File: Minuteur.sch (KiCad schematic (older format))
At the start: 44 parts, among them J1 Screw_Terminal_01x02, J2 ICSP, J3 piezo, J4 Conn_01x10, J5 output, J6 Screw_Terminal_01x03, Q1 BC818, SW1 Rotary_Encoder_Switch, SW2 SW_Push_SPDT_2Leds, U1 ATmega328P-AU, U2 LD1117S50TR_SOT223, U3 MAX7219, U4 PC817, U5 CC56-12EWA, Y1 16MHz

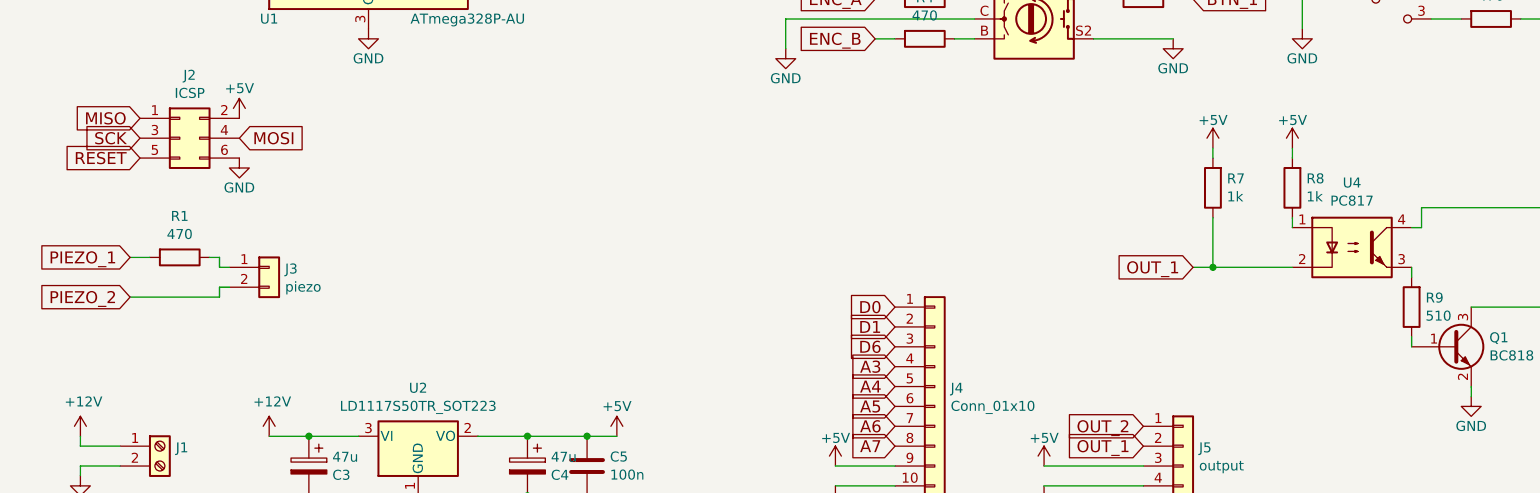
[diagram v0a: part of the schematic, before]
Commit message: All routing done, DRC ok.
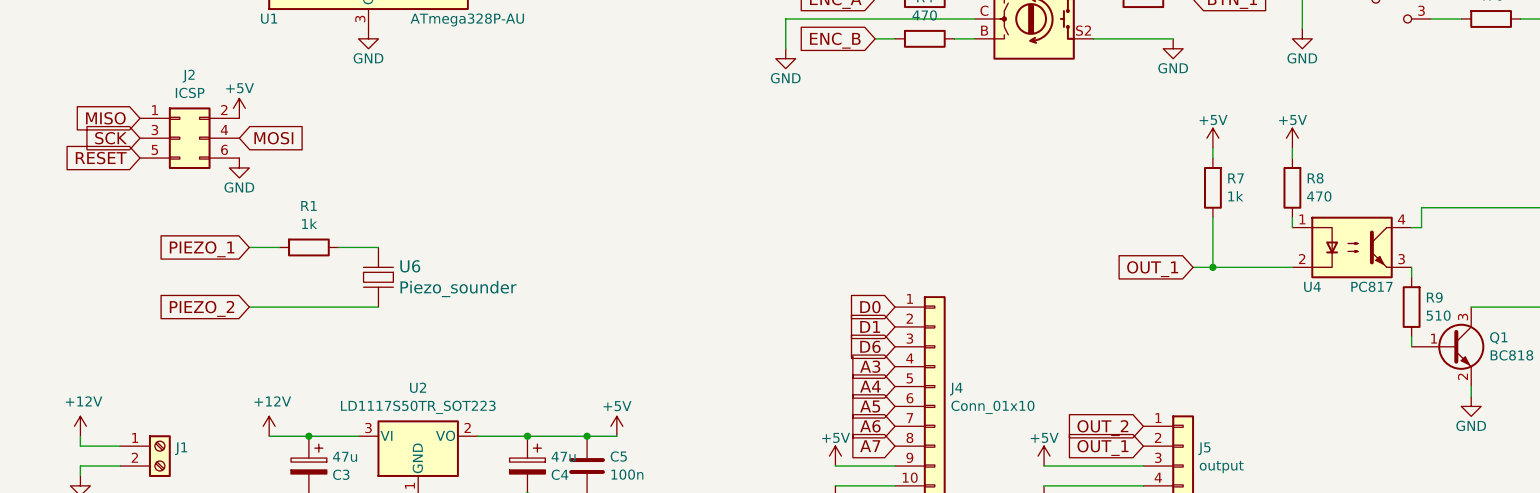
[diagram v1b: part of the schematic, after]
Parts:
- removed J3: piezo, Connector_PinHeader_2.54mm:PinHeader_1x02_P2.54mm_Vertical, symbol Connector_Generic:Conn_01x02
- added U6: Piezo_sounder, IC_Perso:Murata_PKMCS0909_xxxxx, symbol Chip_Perso:Piezo_sounder
- R1: value 470 -> 1k
- R8: value 1k -> 470
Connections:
- net PIEZO_2: now also U6.2
- net at R1.1: now also U6.1
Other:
- moved on the sheet: R1
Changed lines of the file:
@@
 Text GLabel 3150 1700 2    60   Input ~ 0
 PIEZO_2
-Text GLabel 1350 5450 0    60   Input ~ 0
+Text GLabel 1950 5400 0    60   Input ~ 0
 PIEZO_1
 Text GLabel 3150 3700 2    60   Input ~ 0
@@
 	1    0    0    -1
 $EndComp
-Text GLabel 1350 5650 0    60   Input ~ 0
+Text GLabel 1950 5700 0    60   Input ~ 0
 PIEZO_2
 Wire Wire Line
@@
 Wire Wire Line
 	4950 2200 4950 2550
-Wire Wire Line
-	1350 5650 1800 5650
-Wire Wire Line
-	1800 5650 1800 5600
-Wire Wire Line
-	1800 5600 1850 5600
-Wire Wire Line
-	1350 5450 1450 5450
-Wire Wire Line
-	1750 5450 1800 5450
-Wire Wire Line
-	1800 5450 1800 5500
-Wire Wire Line
-	1800 5500 1850 5500
 Text GLabel 3150 1800 2    60   Input ~ 0
 PIEZO_1
@@
 P 7200 5100
 F 0 "R8" H 7130 5054 50  0000 R CNN
-F 1 "1k" H 7130 5145 50  0000 R CNN
+F 1 "470" H 7130 5145 50  0000 R CNN
 F 2 "Resistor_SMD:R_0805_2012Metric" V 7130 5100 50  0001 C CNN
 F 3 "~" H 7200 5100 50  0001 C CNN
@@
 Connection ~ 9100 5200
 $Comp
-L Device:R R1
-U 1 1 5EF81C42
-P 1600 5450
-F 0 "R1" V 1393 5450 50  0000 C CNN
-F 1 "470" V 1484 5450 50  0000 C CNN
-F 2 "Resistor_SMD:R_0805_2012Metric" V 1530 5450 50  0001 C CNN
-F 3 "~" H 1600 5450 50  0001 C CNN
-	1    1600 5450
-	0    1    1    0
-$EndComp
-$Comp
 L Device:C C5
 U 1 1 5EF86361
@@
 U 1 1 5EFADC83
 P 7500 5400
-F 0 "U4" H 7500 5725 50  0000 C CNN
-F 1 "PC817" H 7500 5634 50  0000 C CNN
+F 0 "U4" H 7300 5200 50  0000 C CNN
+F 1 "PC817" H 7600 5200 50  0000 C CNN
 F 2 "Package_DIP:DIP-4_W7.62mm" H 7300 5200 50  0001 L CIN
 F 3 "http://www.soselectronic.cz/a_info/resource/d/pc817.pdf" H 7500 5400 50  0001 L CNN
@@
 	1050 1600 1350 1600
 $Comp
-L Connector_Generic:Conn_01x02 J3
-U 1 1 5EFB8BD6
-P 2050 5500
-F 0 "J3" H 2130 5492 50  0000 L CNN
-F 1 "piezo" H 2130 5401 50  0000 L CNN
-F 2 "Connector_PinHeader_2.54mm:PinHeader_1x02_P2.54mm_Vertical" H 2050 5500 50  0001 C CNN
-F 3 "~" H 2050 5500 50  0001 C CNN
-	1    2050 5500
-	1    0    0    -1
+L Device:R R1
+U 1 1 5EF81C42
+P 2250 5400
+F 0 "R1" V 2043 5400 50  0000 C CNN
+F 1 "1k" V 2134 5400 50  0000 C CNN
+F 2 "Resistor_SMD:R_0805_2012Metric" V 2180 5400 50  0001 C CNN
+F 3 "~" H 2250 5400 50  0001 C CNN
+	1    2250 5400
+	0    1    1    0
+$EndComp
+Wire Wire Line
+	2400 5400 2600 5400
+Wire Wire Line
+	1950 5700 2600 5700
+Wire Wire Line
+	2100 5400 1950 5400
+$Comp
+L Chip_Perso:Piezo_sounder U6
+U 1 1 5FCD1C61
+P 2600 5550
+F 0 "U6" V 2547 5653 60  0000 L CNN
+F 1 "Piezo_sounder" V 2653 5653 60  0000 L CNN
+F 2 "IC_Perso:Murata_PKMCS0909_xxxxx" H 2600 5550 60  0001 C CNN
+F 3 "https://www.murata.com/en-us/products/sound/sounder/pkmcs" H 2600 5550 60  0001 C CNN
+	1    2600 5550
+	0    1    1    0
 $EndComp
 $EndSCHEMATC
